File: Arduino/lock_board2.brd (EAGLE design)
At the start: 14 parts

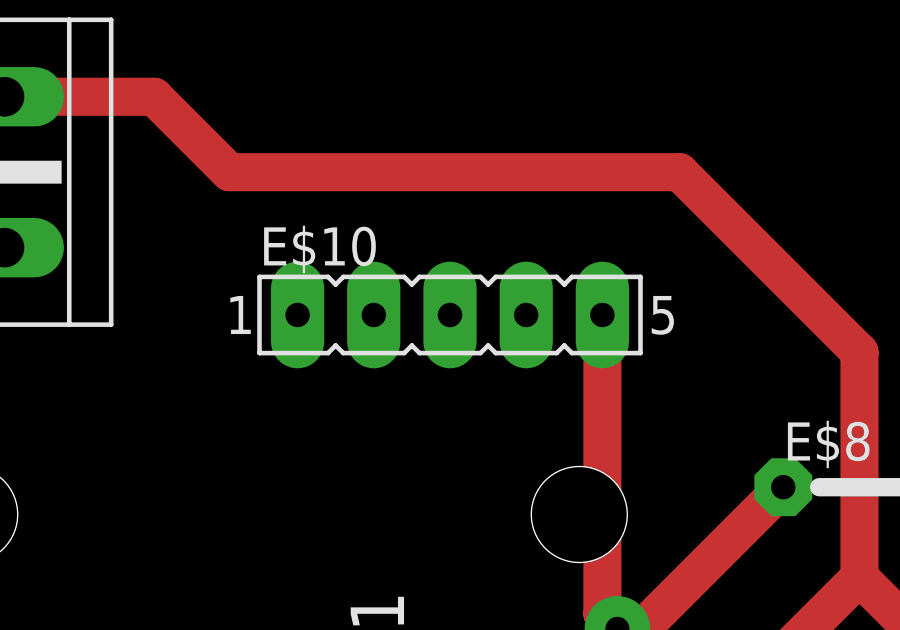
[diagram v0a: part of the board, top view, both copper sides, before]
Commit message: code with token
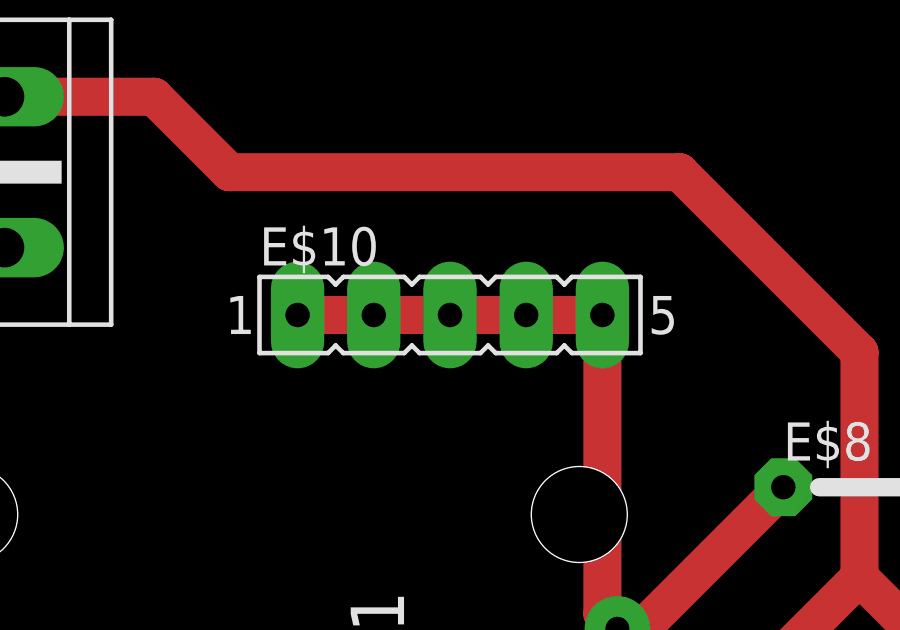
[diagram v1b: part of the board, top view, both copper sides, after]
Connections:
- net S$10: now also E$10.1, E$10.2, E$10.3, E$10.4
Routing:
- net S$10: track 18.2 -> 28.3 mm
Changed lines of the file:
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@@
 <wire x1="47.08" y1="82.5" x2="47.08" y2="72.54" width="1.27" layer="1"/>
 <wire x1="47.08" y1="72.54" x2="47.58" y2="72.04" width="1.27" layer="1"/>
+<contactref element="E$10" pad="4"/>
+<contactref element="E$10" pad="3"/>
+<contactref element="E$10" pad="2"/>
+<contactref element="E$10" pad="1"/>
+<wire x1="36.92" y1="82.5" x2="47.08" y2="82.5" width="1.27" layer="1"/>
+<wire x1="42" y1="82.5" x2="44.54" y2="82.5" width="0" layer="19" extent="1-1"/>
+<wire x1="39.46" y1="82.5" x2="42" y2="82.5" width="0" layer="19" extent="1-1"/>
+<wire x1="47.08" y1="82.5" x2="44.54" y2="82.5" width="0" layer="19" extent="1-1"/>
 </signal>
 <signal name="S$22">
